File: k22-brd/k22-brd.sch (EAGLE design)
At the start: 30 parts, among them IC1 LMS8117, J1 61302011121, J2 61302011121, J3 CORTEX_DEBUG_PTH, SW1 KMR731NGLFS

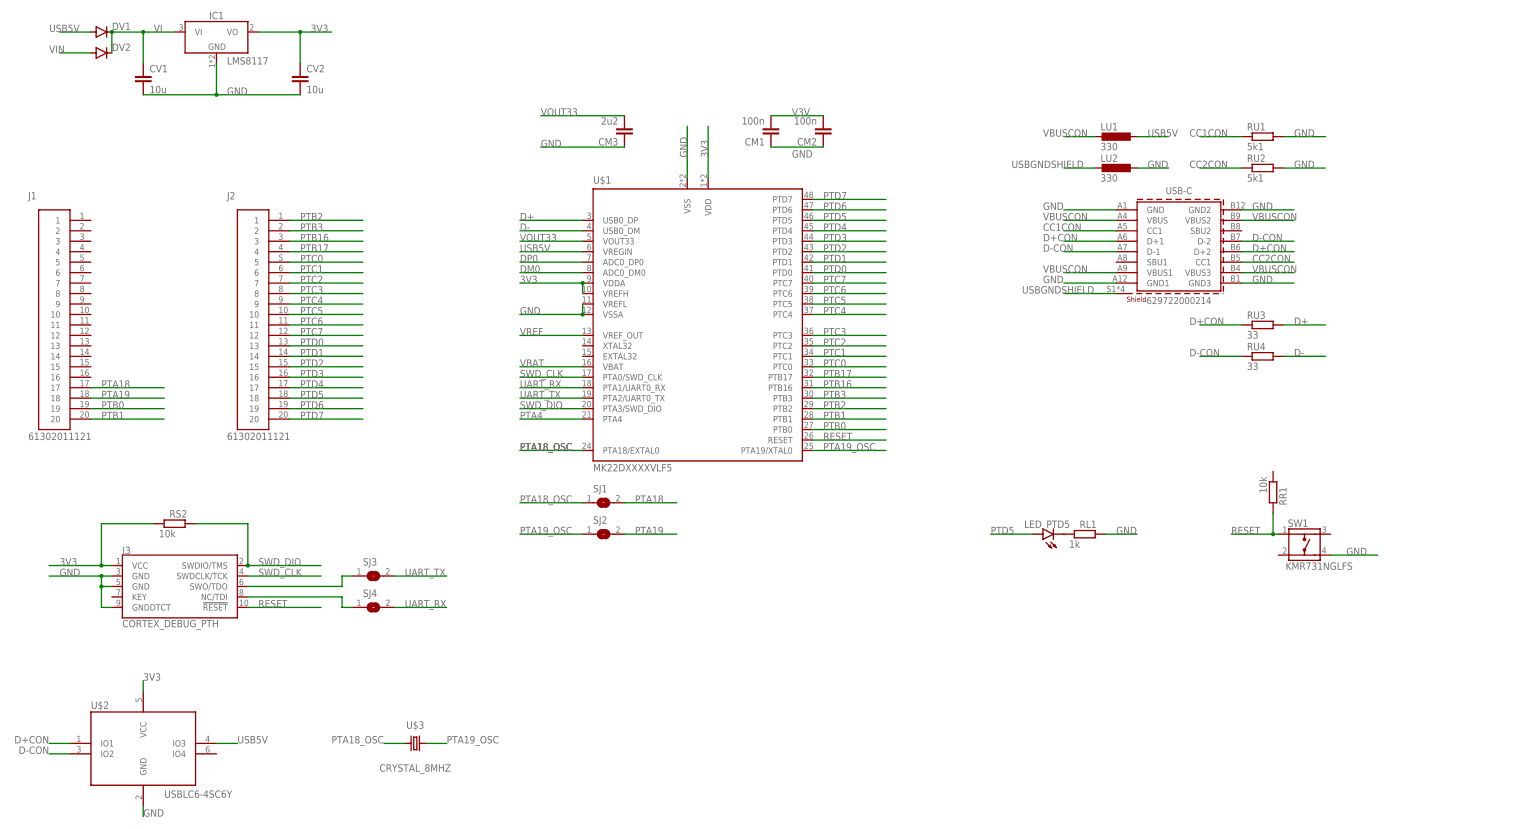
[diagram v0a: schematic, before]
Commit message: schema is done
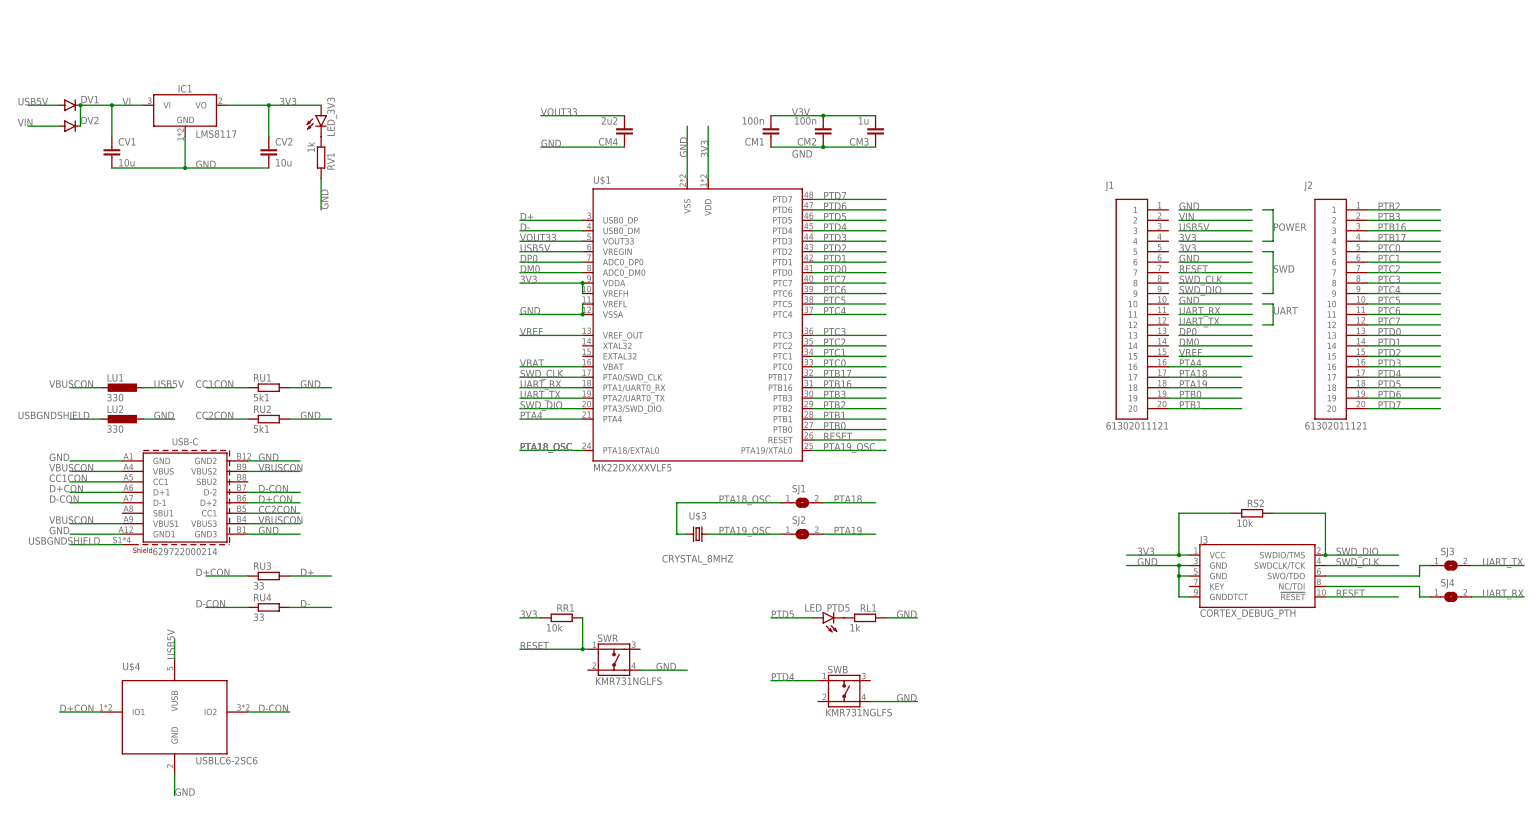
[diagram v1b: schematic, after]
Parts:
- removed SW1: KMR731NGLFS, Switch:KMR731NGLFS
- removed U$2: USBLC6-4SC6Y, vym0038_k22_misc:USBLC6-4SC6Y
- added CM4: 2u2, rcl:C-EUC0805
- added LED_3V3: (no value), led:LEDCHIP-LED0805
- added RV1: 1k, rcl:R-EU_M0805
- added SWB, SWR: KMR731NGLFS, Switch:KMR731NGLFS
- added U$4: USBLC6-2SC6, vym0038_k22_misc:USBLC6-2SC6
- CM3: value 2u2 -> 1u
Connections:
- new net N$2: LED_3V3.C, RV1.1
- net 3V3: now also LED_3V3.A, RR1.1; no longer U$2.VCC
- net D+CON: now also U$4.IO1; no longer U$2.IO1
- net D-CON: now also U$4.IO2; no longer U$2.IO2
- net GND: now also CM4.1, RV1.2, SWB.4, SWR.4, U$4.GND; no longer SW1.4, U$2.GND
- net PTA4: now also J1.16
- net PTD4: now also SWB.1
- net RESET: now also SWR.1; no longer SW1.1
- net USB5V: now also U$4.VUSB; no longer U$2.IO3
- net V3V: now also CM3.2
- net VOUT33: now also CM4.2; no longer CM3.2
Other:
- note added: "B BUTTON PTD4"
- moved on the sheet: CM3, CV1, CV2, DV1, DV2, IC1, J1, J2, J3, LED_PTD5, LU1, LU2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
